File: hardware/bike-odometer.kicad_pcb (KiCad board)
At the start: 2 copper layers, 26 parts, among them J1 Conn_ARM_JTAG_SWD_10, U1 nRF54L05-QFXX, U2 MLX92216, Y1 32 MHz, Y2 32.768 kHz

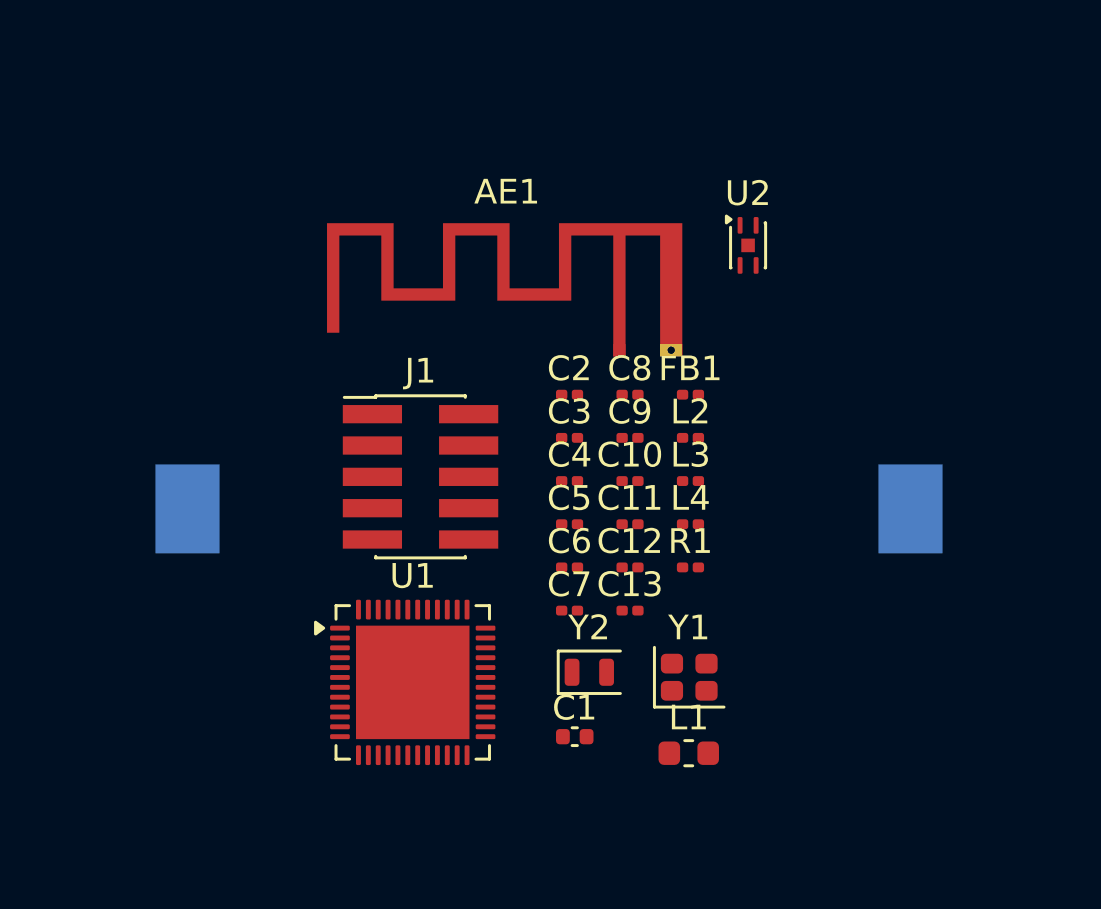
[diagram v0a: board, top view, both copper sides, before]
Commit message: Sourcing complete
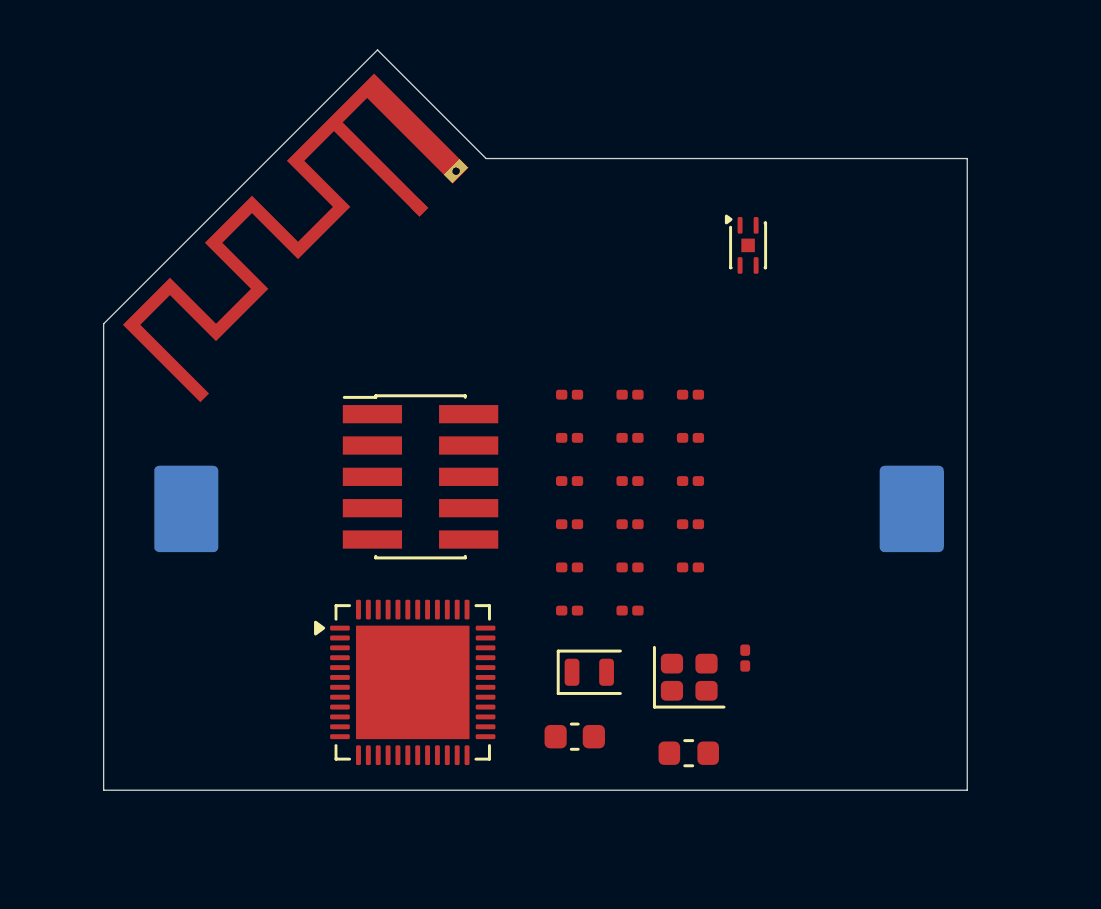
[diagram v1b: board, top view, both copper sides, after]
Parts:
- added C14: 100n, Capacitor_SMD:C_0201_0603Metric, F.Cu at (159.9, 98.9)
- BT1: footprint Battery:BatteryHolder_Keystone_1060_1x2032 -> Battery:BatteryHolder_Renata_SMTU2032-LF_1x2032
- C1: footprint Capacitor_SMD:C_0402_1005Metric -> Capacitor_SMD:C_0603_1608Metric
- moved AE1 9.95 mm to (146.7, 80.7), turned to 45 degrees
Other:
- board outline added: 35 x 30 mm

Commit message: PCB placement
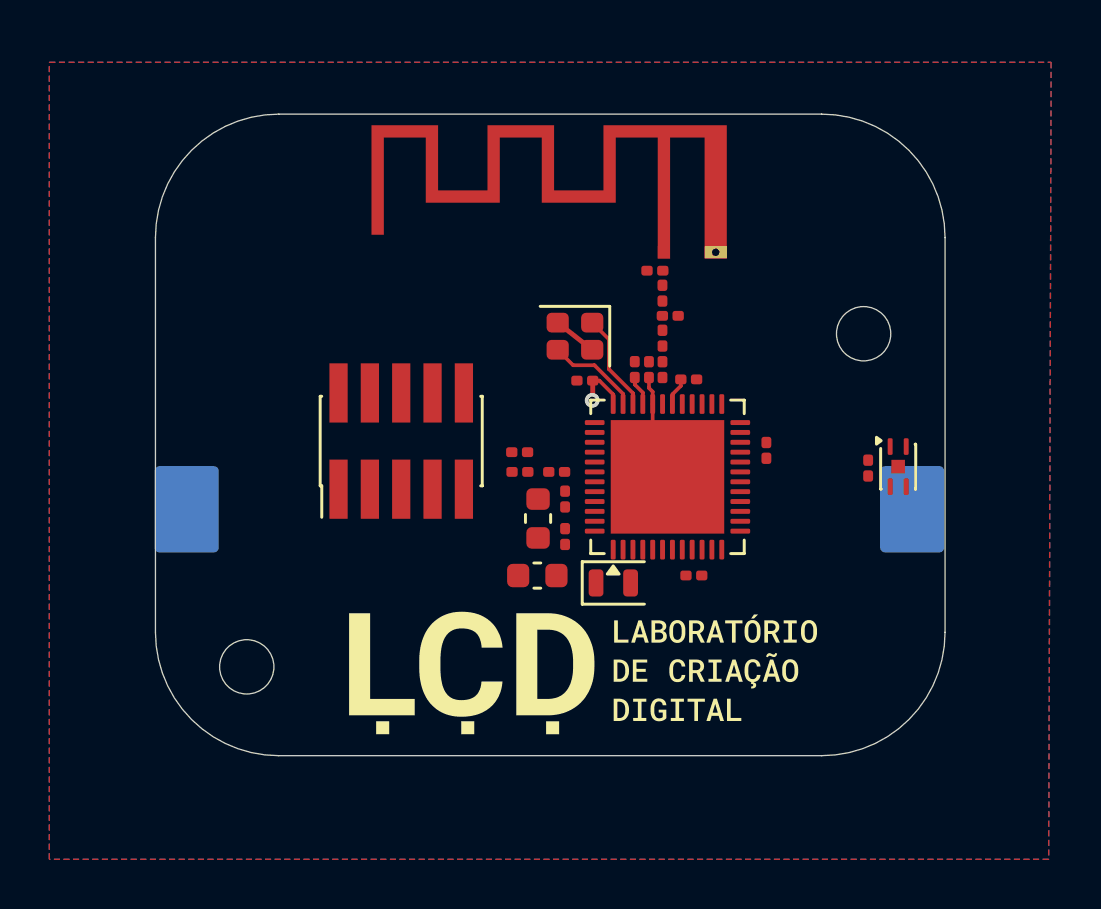
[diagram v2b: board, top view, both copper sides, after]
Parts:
- removed R1: 1k, Resistor_SMD:R_0201_0603Metric
- added H1: MountingHole, MountingHole:MountingHole_2.2mm_M2_ISO14580, F.Cu at (164.7, 85.8)
- added H2: MountingHole, MountingHole:MountingHole_2.2mm_M2_ISO14580, F.Cu at (139.7, 99.3)
- moved Y1 14.6 mm to (153.0, 85.9), turned to 180 degrees
- moved C13 13.8 mm to (156.2, 83.2), turned to 180 degrees
- moved U1 13.3 mm to (156.8, 91.6), turned to 90 degrees
- moved L1 11.3 mm to (151.5, 93.3), turned to 90 degrees
- moved U2 10.8 mm to (166.1, 91.2)
- moved C12 10.3 mm to (156.9, 85.1)
- moved AE1 10.1 mm to (156.6, 82.5), turned to 0 degrees
- moved L4 9.43 mm to (156.5, 84.2), turned to 90 degrees
- moved C14 9.17 mm to (164.9, 91.2)
- moved C5 8.52 mm to (160.8, 90.5), turned to -90 degrees
- moved FB1 7.59 mm to (150.8, 91.4), turned to 180 degrees
- moved C7 6.73 mm to (150.8, 90.6), turned to 180 degrees
- moved C1 6.70 mm to (151.5, 95.6), turned to 180 degrees
- moved C4 6.33 mm to (157.8, 95.6), turned to 180 degrees
- moved C11 6.31 mm to (156.0, 87.3), turned to -90 degrees
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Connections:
- C10 pad 1: Net-(U1-~{RESET}) -> Net-(J1-~{RESET})
- U1 pad 30: Net-(U1-~{RESET}) -> Net-(J1-~{RESET})
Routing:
- net GND: track 0.00 -> 6.12 mm
- net Net-(U1-XC1): track 0.00 -> 3.98 mm
- net Net-(U1-XC2): track 0.00 -> 3.80 mm
- net +BATT: track 0.00 -> 2.26 mm, vias 0 -> 1
- net Net-(U1-DECA): track 0.00 -> 1.21 mm
- net Net-(J1-~{RESET}): track 0.00 -> 1.14 mm
- added copper zone on B.Cu, net GND
- added copper zone on F.Cu, net GND
- added copper zone on In1.Cu, net GND
- added copper zone on In2.Cu, net GND
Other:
- board size 35 x 30 mm -> 32 x 26 mm
- copper layers 2 -> 4
